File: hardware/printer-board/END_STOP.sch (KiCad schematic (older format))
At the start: 27 parts, among them J15 X_MIN, J16 X_MAX, J17 Y_MIN, J18 Y_MAX, J19 Z_MIN, J20 Z_MAX, J45 END_SWITCH_DEBUG, J48 HOTEND_PROBE

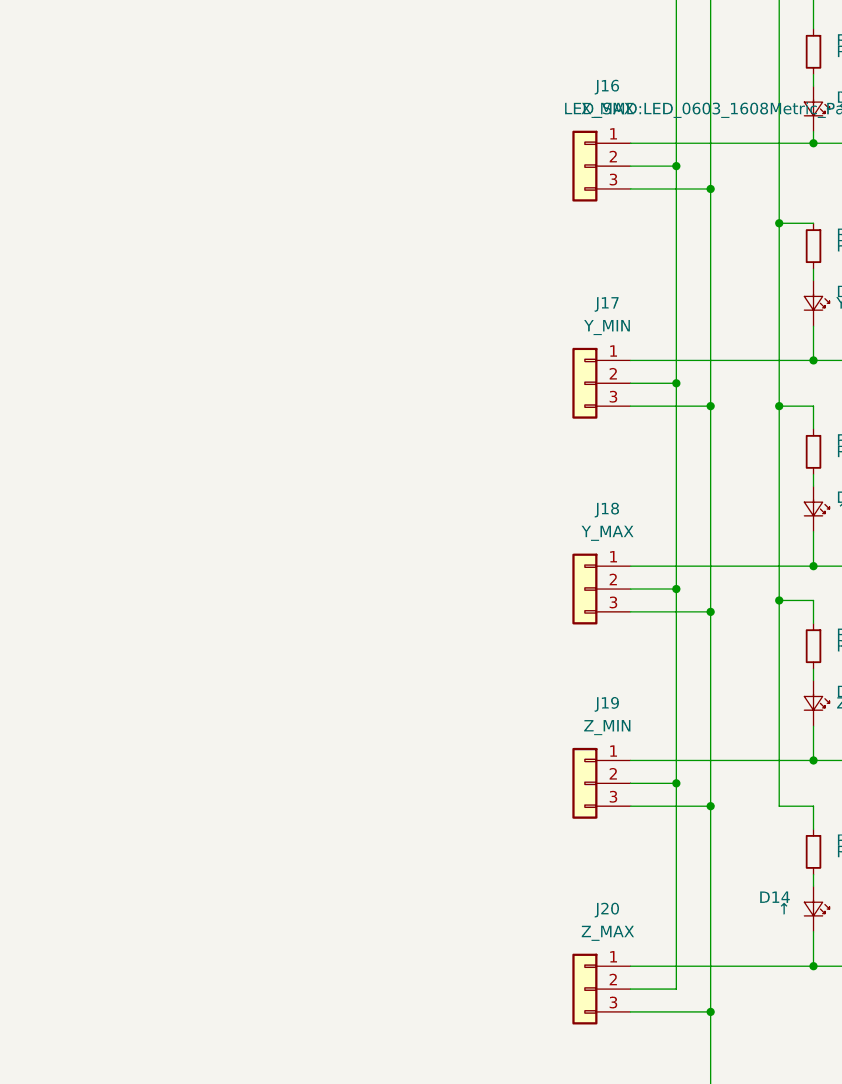
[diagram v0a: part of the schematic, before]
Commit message: update,
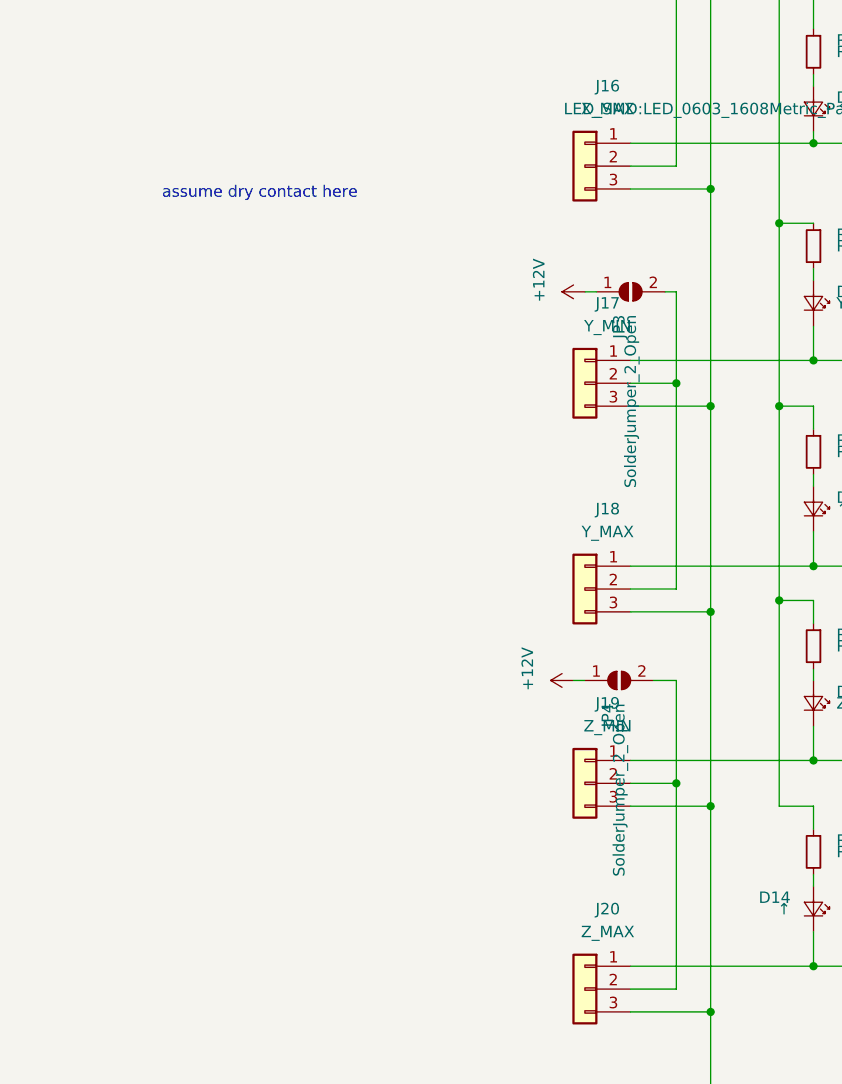
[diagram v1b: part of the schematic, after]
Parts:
- added JP3, JP4: SolderJumper_2_Open, Jumper:SolderJumper-2_P1.3mm_Open_RoundedPad1.0x1.5mm, symbol Jumper:SolderJumper_2_Open
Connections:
- net +12V: now also JP3.1 (A), JP4.1 (A)
- new net: J15.2 (Pin_2), J16.2 (Pin_2), JP1.2 (B)
- new net: J17.2 (Pin_2), J18.2 (Pin_2), JP3.2 (B)
- new net: J19.2 (Pin_2), J20.2 (Pin_2), JP4.2 (B)
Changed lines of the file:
@@
 Wire Wire Line
 	4250 5350 4250 5500
-Wire Wire Line
-	4250 5500 3450 5500
 $Comp
 L taobao-r:R102,0603 R34
@@
 Wire Wire Line
 	3450 2900 3650 2900
-Connection ~ 3650 2900
 Wire Wire Line
 	3450 3000 3800 3000
@@
 Wire Wire Line
 	3450 3850 3650 3850
-Connection ~ 3650 3850
 Wire Wire Line
 	3450 3950 3800 3950
@@
 Wire Wire Line
 	3450 4750 3650 4750
-Connection ~ 3650 4750
 Wire Wire Line
 	3450 4850 3800 4850
@@
 Wire Wire Line
 	3450 5600 3650 5600
-Connection ~ 3650 5600
 Wire Wire Line
 	3450 5700 3800 5700
@@
 	4250 2800 4650 2800
 Wire Wire Line
-	3650 2900 3650 3850
-Wire Wire Line
 	3650 3850 3650 4750
-Wire Wire Line
-	3650 4750 3650 5600
 Wire Wire Line
 	3650 5600 3650 6500
@@
 Wire Wire Line
 	1100 1600 1650 1600
+$Comp
+L power:+12V #PWR0195
+U 1 1 5CD07A9A
+P 3250 3450
+F 0 "#PWR0195" H 3250 3300 50  0001 C CNN
+F 1 "+12V" H 3300 3650 50  0000 C CNN
+F 2 "" H 3250 3450 50  0001 C CNN
+F 3 "" H 3250 3450 50  0001 C CNN
+	1    3250 3450
+	0    -1   -1   0
+$EndComp
+$Comp
+L Jumper:SolderJumper_2_Open JP3
+U 1 1 5CD07AA4
+P 3450 3450
+F 0 "JP3" V 3400 3350 50  0000 R CNN
+F 1 "SolderJumper_2_Open" V 3450 3350 50  0000 R CNN
+F 2 "Jumper:SolderJumper-2_P1.3mm_Open_RoundedPad1.0x1.5mm" H 3450 3450 50  0001 C CNN
+F 3 "~" H 3450 3450 50  0001 C CNN
+	1    3450 3450
+	1    0    0    -1
+$EndComp
+Wire Wire Line
+	3250 3450 3300 3450
+Text Notes 1400 3050 0    50   ~ 0
+assume dry contact here
+Connection ~ 3650 3850
+Wire Wire Line
+	4250 5500 3450 5500
+Wire Wire Line
+	3550 5150 3650 5150
+Wire Wire Line
+	3200 5150 3250 5150
+$Comp
+L Jumper:SolderJumper_2_Open JP4
+U 1 1 5CD18A57
+P 3400 5150
+F 0 "JP4" V 3350 5050 50  0000 R CNN
+F 1 "SolderJumper_2_Open" V 3400 5050 50  0000 R CNN
+F 2 "Jumper:SolderJumper-2_P1.3mm_Open_RoundedPad1.0x1.5mm" H 3400 5150 50  0001 C CNN
+F 3 "~" H 3400 5150 50  0001 C CNN
+	1    3400 5150
+	1    0    0    -1
+$EndComp
+$Comp
+L power:+12V #PWR0196
+U 1 1 5CD18A4D
+P 3200 5150
+F 0 "#PWR0196" H 3200 5000 50  0001 C CNN
+F 1 "+12V" H 3250 5350 50  0000 C CNN
+F 2 "" H 3200 5150 50  0001 C CNN
+F 3 "" H 3200 5150 50  0001 C CNN
+	1    3200 5150
+	0    -1   -1   0
+$EndComp
+Wire Wire Line
+	3650 5150 3650 5600
+Connection ~ 3650 5600
+Wire Wire Line
+	3600 3450 3650 3450
+Wire Wire Line
+	3650 3450 3650 3850
 $EndSCHEMATC
